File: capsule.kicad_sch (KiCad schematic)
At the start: 78 parts, among them J1 OLED-128x128, J2 Conn_01x01_Socket, SW1 SW, SW10 SW, SW11 SW, SW12 SW, SW13 SW, SW14 SW, SW15 SW, SW16 SW, SW17 SW, SW18 SW, SW19 SW, SW2 SW, SW20 SW, SW21 SW, SW22 SW, SW23 SW, SW24 SW, SW25 SW, SW26 SW, SW27 SW, SW28 SW, SW29 SW, SW3 SW, SW30 SW, SW4 SW, SW5 SW, SW6 SW, SW7 SW, SW8 SW, SW9 SW, U1 ProMicro

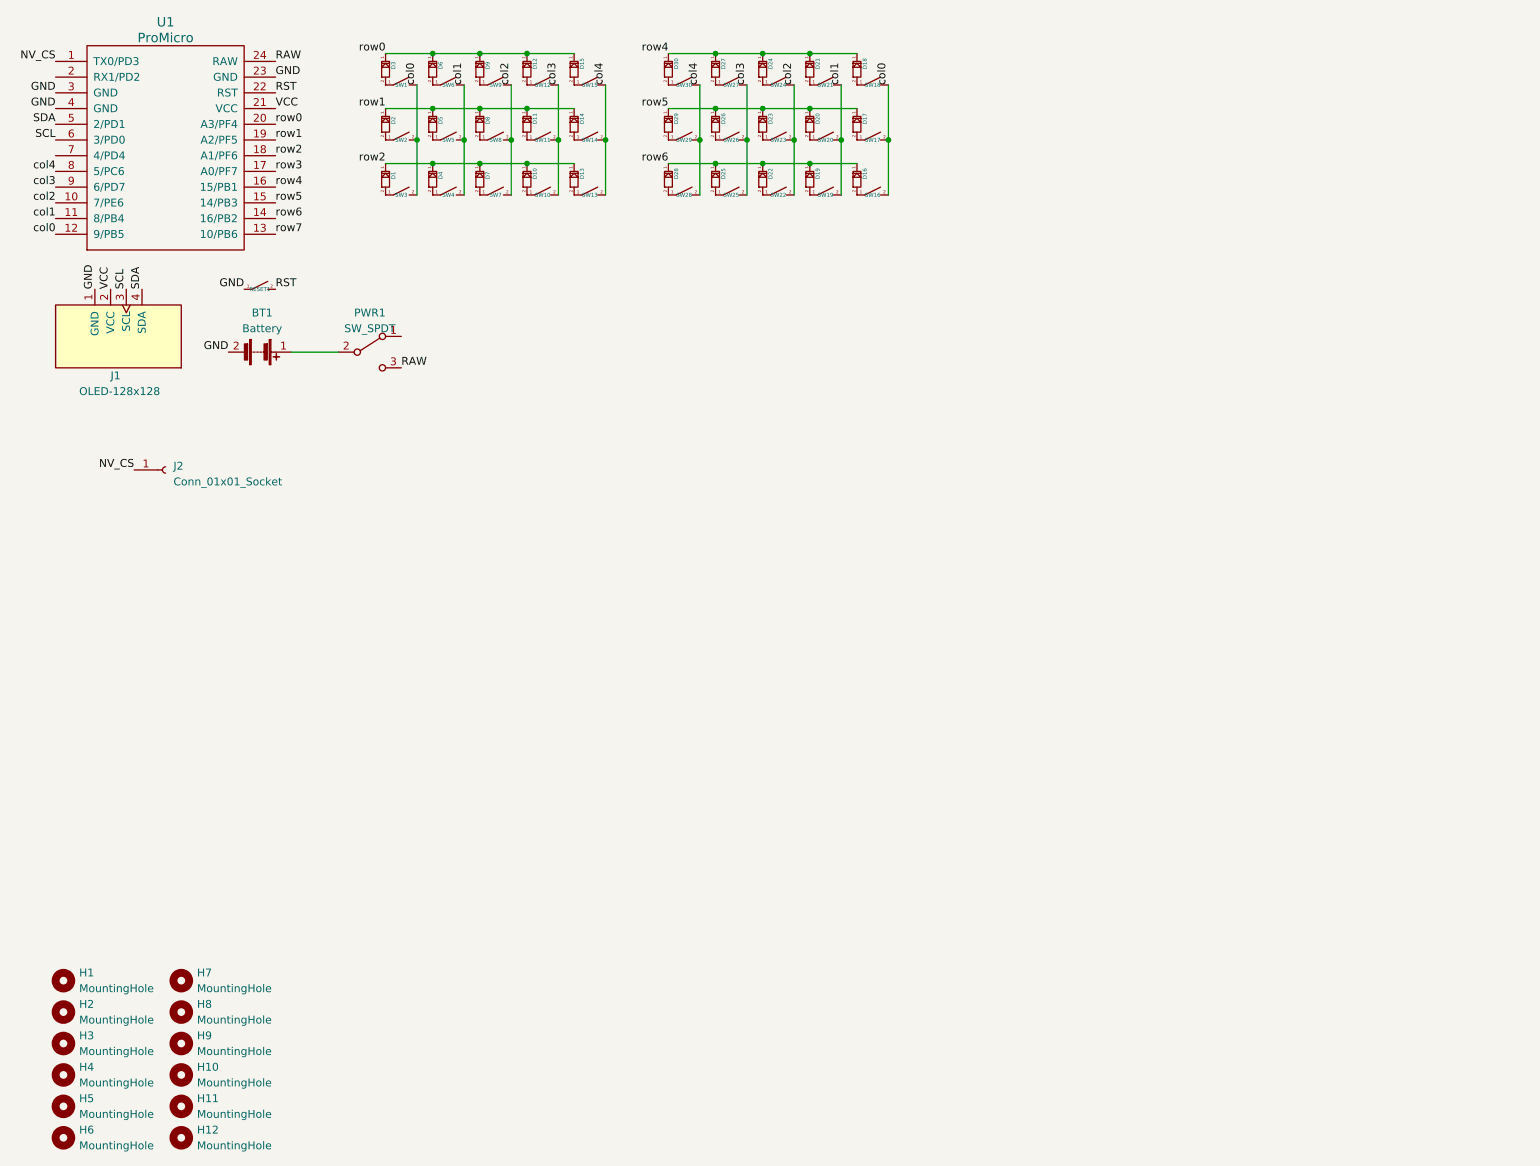
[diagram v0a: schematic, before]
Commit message: sch refactor
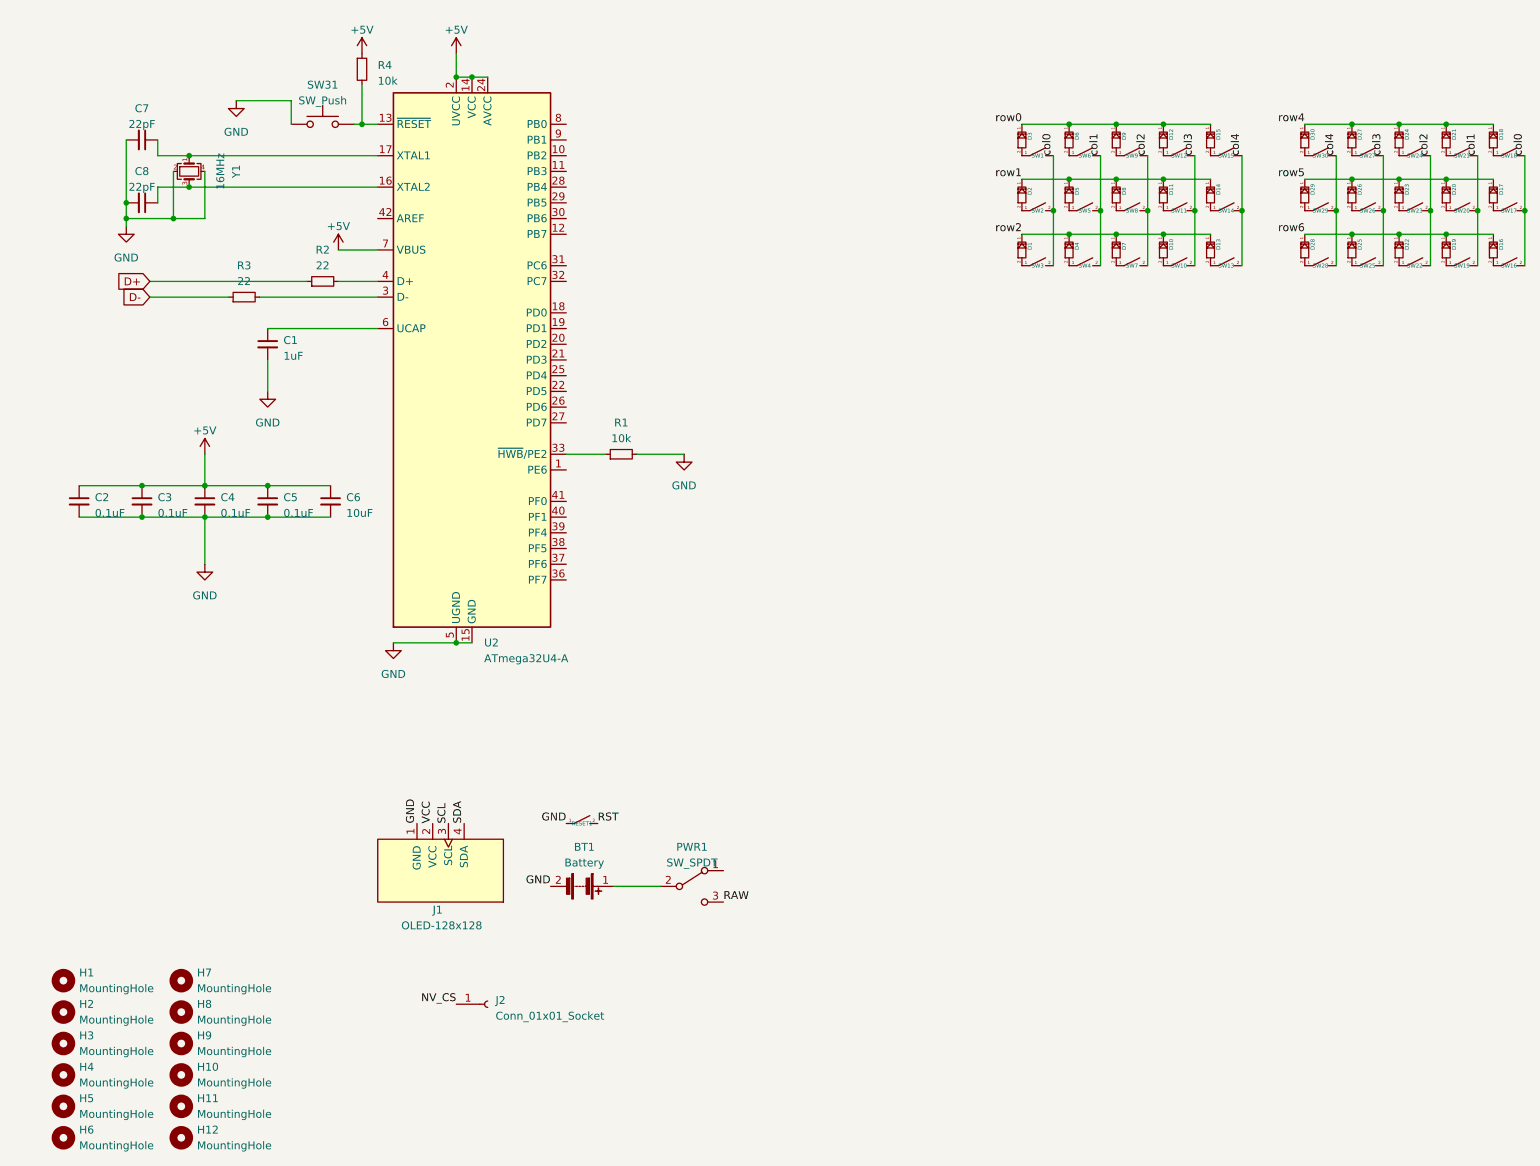
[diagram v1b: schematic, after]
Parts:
- removed U1: ProMicro, Keebio-Parts:ArduinoProMicro, symbol keebio:ProMicro
- added C1: 1uF, symbol Device:C_Small
- added C2, C3, C4, C5: 0.1uF, symbol Device:C_Small
- added C6: 10uF, symbol Device:C_Small
- added C7, C8: 22pF, symbol Device:C_Small
- added R1, R4: 10k, symbol Device:R_Small
- added R2, R3: 22, symbol Device:R_Small
- added SW31: SW_Push, symbol Switch:SW_Push
- added U2: ATmega32U4-A, Package_QFP:TQFP-44_10x10mm_P0.8mm, symbol MCU_Microchip_ATmega:ATmega32U4-A
- added Y1: 16MHz, symbol Device:Crystal_GND24_Small
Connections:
- net GND: now also C1.2, C2.2, C3.2, C4.2, C5.2, C6.2, C7.2, C8.2, R1.2, SW31.1, U2.15 (GND), U2.23 (GND), U2.35 (GND), U2.43 (GND), U2.5 (UGND), Y1.2, Y1.4
- new net: R1.1, U2.33 (~{HWB}/PE2)
- new net: C7.1, U2.17 (XTAL1), Y1.1
- new net: C8.1, U2.16 (XTAL2), Y1.3
- new net: R2.2, U2.4 (D+)
- new net: R4.2, SW31.2, U2.13 (~{RESET})
- new net: R3.2, U2.3 (D-)
- new net: C1.1, U2.6 (UCAP)
- new net +5V: C2.1, C3.1, C4.1, C5.1, C6.1, R4.1, U2.14 (VCC), U2.2 (UVCC), U2.24 (AVCC), U2.34 (VCC), U2.44 (AVCC), U2.7 (VBUS)
- new net D+: R2.1
- new net D-: R3.1
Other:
- moved on the sheet: BT1, D1, D10, D11, D12, D13, D14, D15, D16, D17, D18, D19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
